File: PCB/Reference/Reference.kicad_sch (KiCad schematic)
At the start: 31 parts, among them J1 Conn_01x04, U1 LMR16006XDDCR, U2 Barcode, U2 MD8942

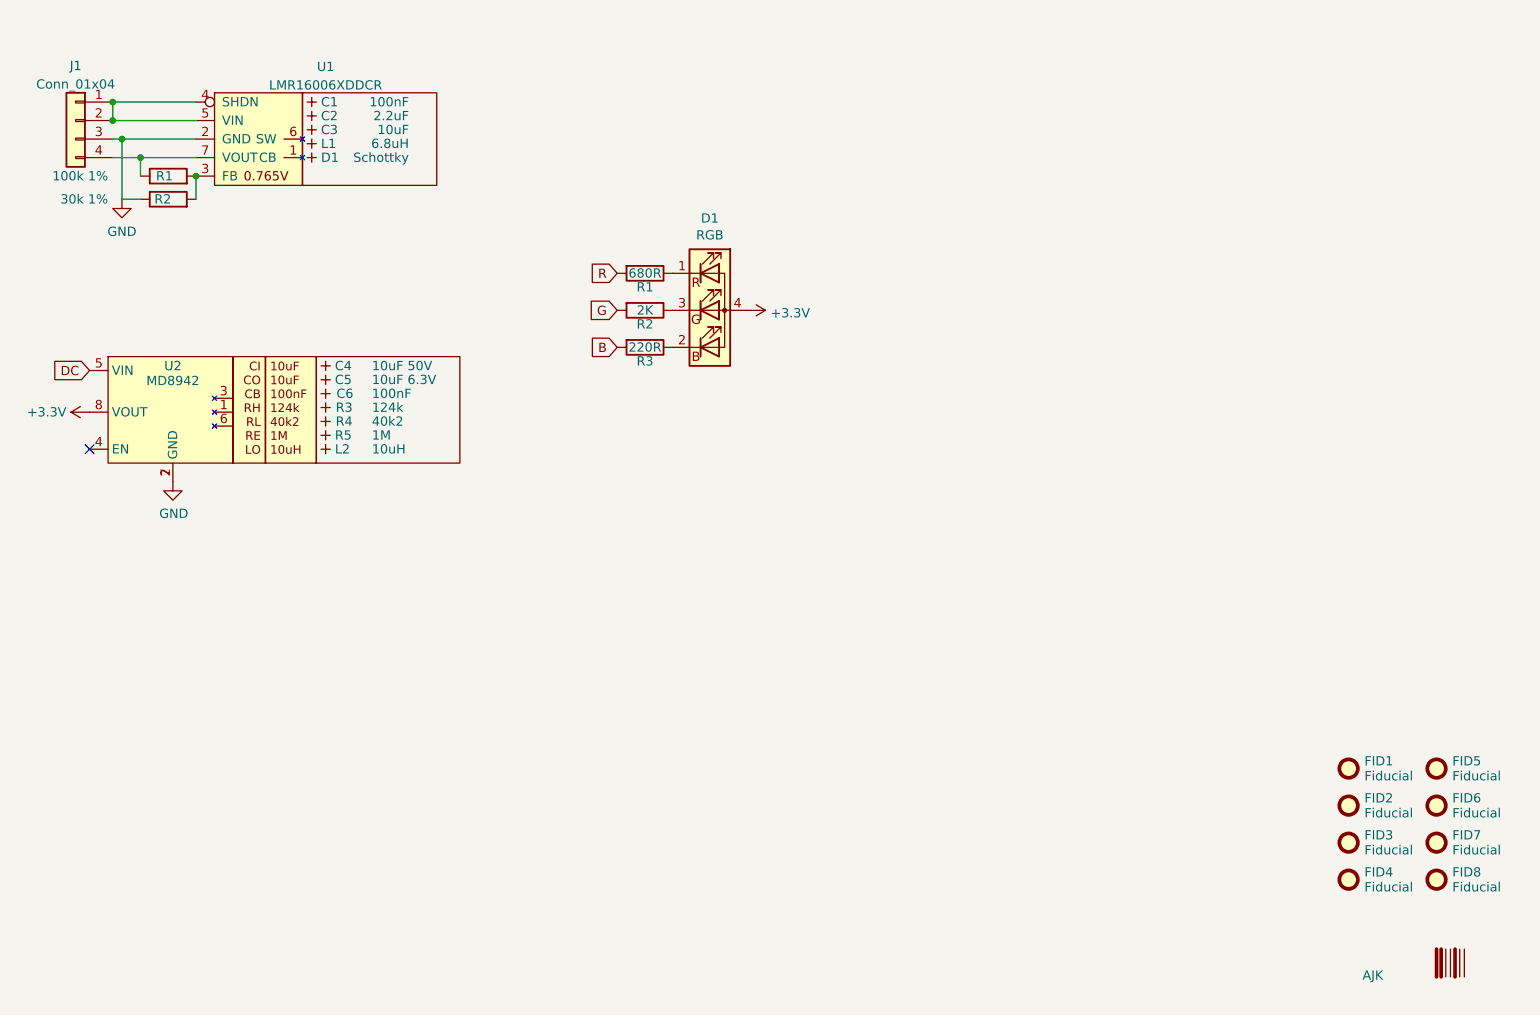
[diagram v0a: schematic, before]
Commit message: PCB templatge
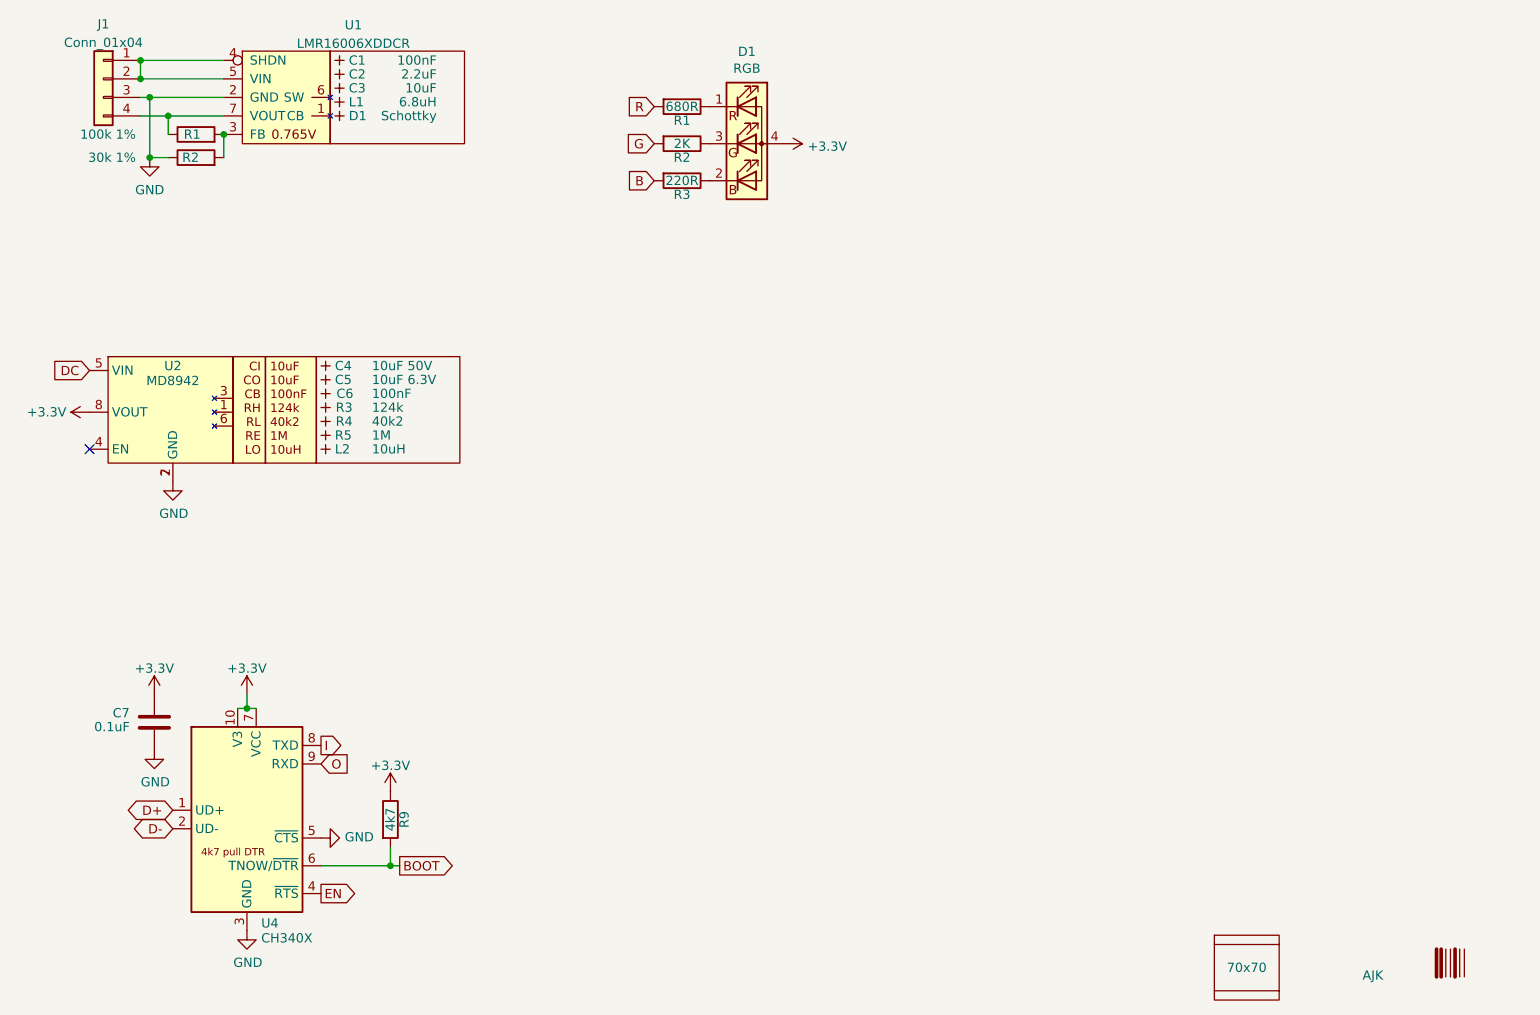
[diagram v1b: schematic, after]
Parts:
- removed FID1, FID2, FID3, FID4, FID5, FID6, FID7, FID8: Fiducial, Fiducial:Fiducial_1mm_Mask2mm, symbol Mechanical:Fiducial
- added C7: 0.1uF, RevK:C_0402, symbol Device:C
- added PCB1: 70x70, RevK:PCB7070, symbol RevK:PCB
- added R9: 4k7, RevK:R_0402, symbol Device:R
- added U4: CH340X, RevK:CH340X, symbol RevK:CH340X
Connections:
- net +3.3V: now also C7.1, R9.1, U4.10 (V3), U4.7 (VCC)
- net GND: now also C7.2, U4.3 (GND), U4.5 (~{CTS})
- new net BOOT: R9.2, U4.6 (TNOW/~{DTR})
- new net D+: U4.1 (UD+)
- new net D-: U4.2 (UD-)
- new net EN: U4.4 (~{RTS})
- new net I: U4.8 (TXD)
- new net O: U4.9 (RXD)
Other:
- moved on the sheet: C1, C2, C3, D1, J1, L1, R1, R2, R3, U1
